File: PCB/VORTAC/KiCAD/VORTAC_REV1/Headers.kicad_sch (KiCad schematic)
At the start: 7 parts, among them J1 DEBUG, J14 918-418K2023S40001, J15 STEPPER, J3 Conn_01x05

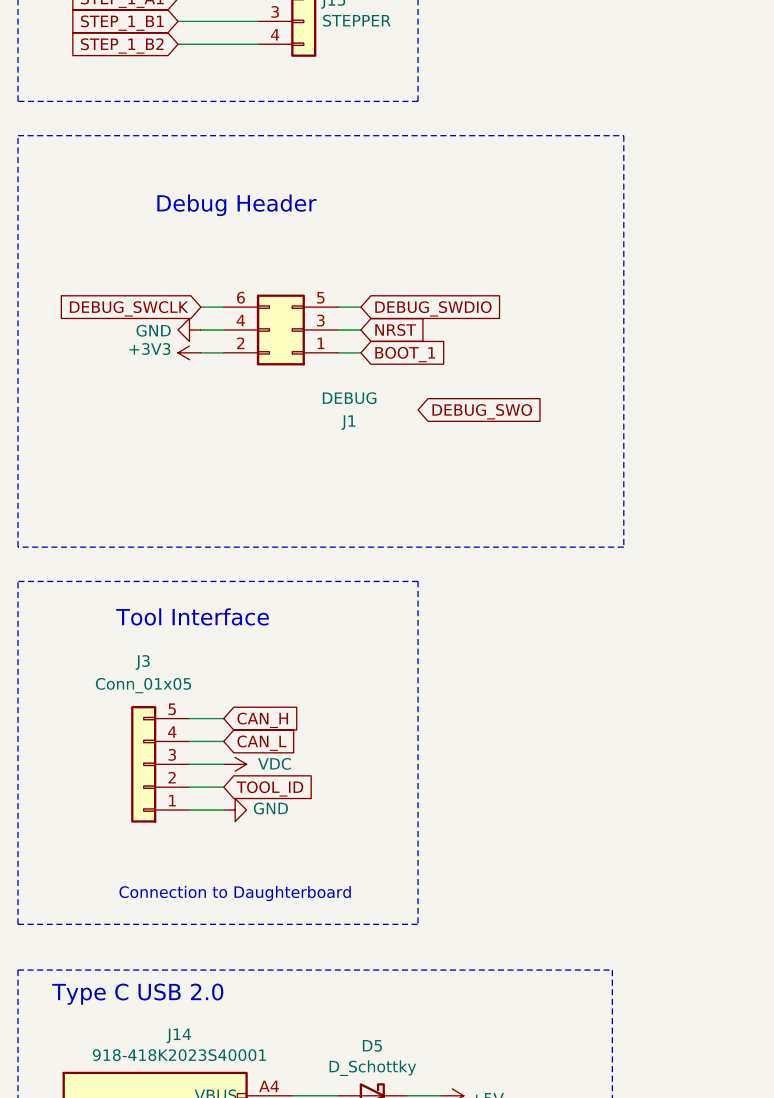
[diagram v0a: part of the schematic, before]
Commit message: Wayollaaaaa
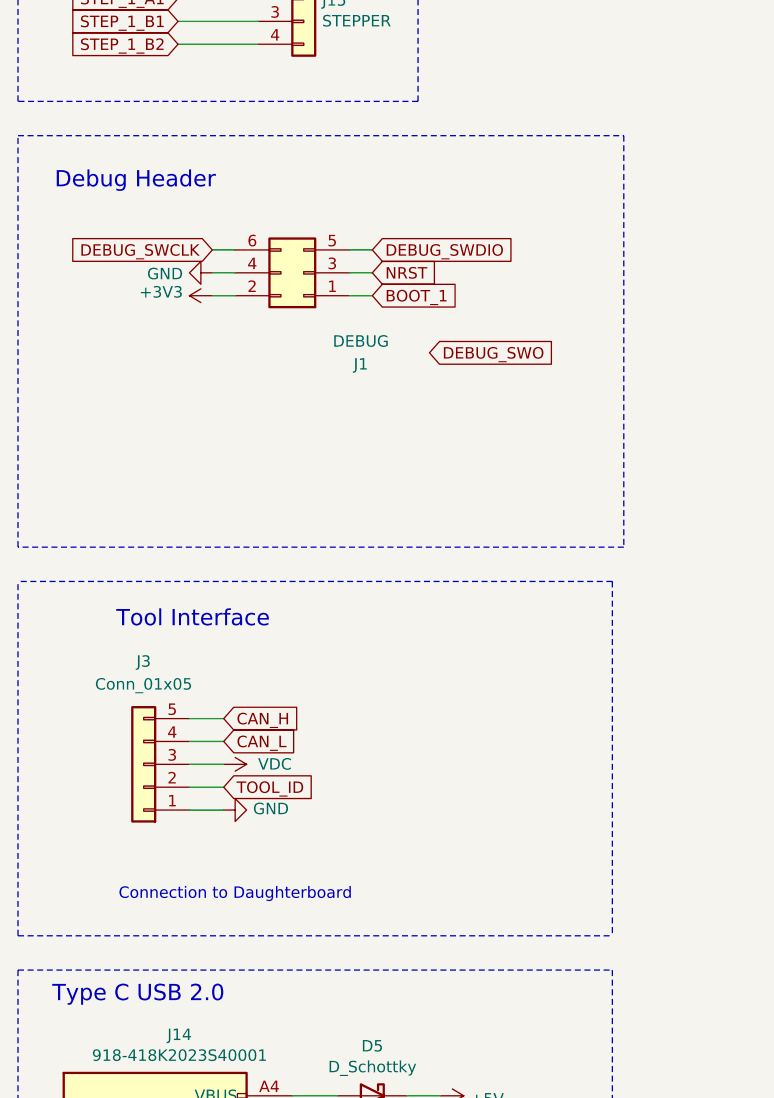
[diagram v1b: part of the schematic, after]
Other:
- moved on the sheet: J1
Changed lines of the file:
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@@
 	(polyline
 		(pts
-			(xy 16.51 132.08) (xy 16.51 93.98)
+			(xy 16.51 133.35) (xy 16.51 93.98)
 		)
 		(stroke
@@
 	(polyline
 		(pts
-			(xy 60.96 93.98) (xy 60.96 132.08)
+			(xy 82.55 93.98) (xy 82.55 133.35)
 		)
 		(stroke
@@
 	(polyline
 		(pts
-			(xy 60.96 93.98) (xy 16.51 93.98)
+			(xy 82.55 93.98) (xy 16.51 93.98)
 		)
 		(stroke
@@
 	(wire
 		(pts
-			(xy 36.83 63.5) (xy 39.37 63.5)
-		)
-		(stroke
-			(width 0)
-			(type default)
-		)
-	)
-	(wire
-		(pts
-			(xy 54.61 68.58) (xy 52.07 68.58)
+			(xy 38.1 57.15) (xy 40.64 57.15)
+		)
+		(stroke
+			(width 0)
+			(type default)
+		)
+	)
+	(wire
+		(pts
+			(xy 55.88 62.23) (xy 53.34 62.23)
 		)
 		(stroke
@@
 	(wire
 		(pts
-			(xy 52.07 63.5) (xy 54.61 63.5)
-		)
-		(stroke
-			(width 0)
-			(type default)
-		)
-	)
-	(wire
-		(pts
-			(xy 39.37 66.04) (xy 36.83 66.04)
+			(xy 53.34 57.15) (xy 55.88 57.15)
+		)
+		(stroke
+			(width 0)
+			(type default)
+		)
+	)
+	(wire
+		(pts
+			(xy 40.64 59.69) (xy 38.1 59.69)
 		)
 		(stroke
@@
 	(wire
 		(pts
-			(xy 52.07 66.04) (xy 54.61 66.04)
+			(xy 53.34 59.69) (xy 55.88 59.69)
 		)
 		(stroke
@@
 	(polyline
 		(pts
-			(xy 16.51 132.08) (xy 60.96 132.08)
+			(xy 16.51 133.35) (xy 82.55 133.35)
 		)
 		(stroke
@@
 	(wire
 		(pts
-			(xy 36.83 68.58) (xy 39.37 68.58)
+			(xy 38.1 62.23) (xy 40.64 62.23)
 		)
 		(stroke
@@
 	(text "Debug Header"
 		(exclude_from_sim no)
-		(at 31.75 53.34 0)
+		(at 20.574 50.546 0)
 		(effects
 			(font
@@
 	(global_label "BOOT_1"
 		(shape input)
-		(at 54.61 68.58 0)
+		(at 55.88 62.23 0)
 		(effects
 			(font
@@
 		)
 		(property "Intersheetrefs" "${INTERSHEET_REFS}"
-			(at 54.61 68.58 0)
+			(at 55.88 62.23 0)
 			(effects
 				(font
@@
 	(global_label "DEBUG_SWDIO"
 		(shape input)
-		(at 54.61 63.5 0)
+		(at 55.88 57.15 0)
 		(effects
 			(font
@@
 		)
 		(property "Intersheetrefs" "${INTERSHEET_REFS}"
-			(at 54.61 63.5 0)
+			(at 55.88 57.15 0)
 			(effects
 				(font
@@
 	(global_label "NRST"
 		(shape input)
-		(at 54.61 66.04 0)
+		(at 55.88 59.69 0)
 		(effects
 			(font
@@
 		)
 		(property "Intersheetrefs" "${INTERSHEET_REFS}"
-			(at 54.61 66.04 0)
+			(at 55.88 59.69 0)
 			(effects
 				(font
@@
 	(global_label "DEBUG_SWO"
 		(shape input)
-		(at 60.96 74.93 0)
+		(at 62.23 68.58 0)
 		(effects
 			(font
@@
 		)
 		(property "Intersheetrefs" "${INTERSHEET_REFS}"
-			(at 60.96 74.93 0)
+			(at 62.23 68.58 0)
 			(effects
 				(font
@@
 	(global_label "DEBUG_SWCLK"
 		(shape input)
-		(at 36.83 63.5 180)
+		(at 38.1 57.15 180)
 		(effects
 			(font
@@
 		)
 		(property "Intersheetrefs" "${INTERSHEET_REFS}"
-			(at 36.83 63.5 0)
+			(at 38.1 57.15 0)
 			(effects
 				(font
@@
 	(symbol
 		(lib_id "Connector_Generic:Conn_02x03_Odd_Even")
-		(at 46.99 66.04 180)
+		(at 48.26 59.69 180)
 		(unit 1)
 		(exclude_from_sim no)
@@
 		(dnp no)
 		(property "Reference" "J1"
-			(at 53.34 76.2 0)
+			(at 54.61 69.85 0)
 			(effects
 				(font
@@
 		)
 		(property "Value" "DEBUG"
-			(at 53.34 73.66 0)
+			(at 54.61 67.31 0)
 			(effects
 				(font
@@
 		)
 		(property "Footprint" "ToolChanger:PinHeader_2x03_P1.27mm_Vertical"
-			(at 46.99 66.04 0)
+			(at 48.26 59.69 0)
 			(effects
 				(font
@@
 		)
 		(property "Datasheet" "~"
-			(at 46.99 66.04 0)
+			(at 48.26 59.69 0)
 			(effects
 				(font
@@
 		)
 		(property "Description" "Generic connector, double row, 02x03, odd/even pin numbering scheme (row 1 odd numbers, row 2 even numbers), script generated (kicad-library-utils/schlib/autogen/connector/)"
-			(at 46.99 66.04 0)
+			(at 48.26 59.69 0)
 			(effects
 				(font
@@
 	(symbol
 		(lib_id "VORTAC-rescue:+3.3V-power")
-		(at 36.83 68.58 90)
+		(at 38.1 62.23 90)
 		(unit 1)
 		(exclude_from_sim no)
@@
 		(dnp no)
 		(property "Reference" "#PWR0160"
-			(at 40.64 68.58 0)
+			(at 41.91 62.23 0)
 			(effects
 				(font
@@
 		)
 		(property "Value" "+3V3"
-			(at 33.5788 68.199 90)
+			(at 34.8488 61.849 90)
 			(effects
 				(font
@@
 		)
 		(property "Footprint" ""
-			(at 36.83 68.58 0)
+			(at 38.1 62.23 0)
 			(effects
 				(font
@@
 		)
 		(property "Datasheet" ""
-			(at 36.83 68.58 0)
+			(at 38.1 62.23 0)
 			(effects
 				(font
@@
 		)
 		(property "Description" ""
-			(at 36.83 68.58 0)
+			(at 38.1 62.23 0)
 			(effects
 				(font
@@
 	(symbol
 		(lib_id "VORTAC-rescue:GND-power")
-		(at 36.83 66.04 270)
+		(at 38.1 59.69 270)
 		(unit 1)
 		(exclude_from_sim no)
@@
 		(dnp no)
 		(property "Reference" "#PWR0161"
-			(at 30.48 66.04 0)
+			(at 31.75 59.69 0)
 			(effects
 				(font
@@
 		)
 		(property "Value" "GND"
-			(at 33.5788 66.167 90)
+			(at 34.8488 59.817 90)
 			(effects
 				(font
@@
 		)
 		(property "Footprint" ""
-			(at 36.83 66.04 0)
+			(at 38.1 59.69 0)
 			(effects
 				(font
@@
 		)
 		(property "Datasheet" ""
-			(at 36.83 66.04 0)
+			(at 38.1 59.69 0)
 			(effects
 				(font
@@
 		)
 		(property "Description" ""
-			(at 36.83 66.04 0)
-			(effects
-				(font
+			(at 38.1 59.69 0)
+			(effects
+				(font

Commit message: Fixed Library stuff
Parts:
- J1: footprint ToolChanger:PinHeader_2x03_P1.27mm_Vertical -> Vortac:PinHeader_2x03_P1.27mm_Vertical
- J14: footprint ToolChanger:USB-C-TH_HANBO_MC-118LD-H65 -> Vortac:USB-C-TH_HANBO_MC-118LD-H65
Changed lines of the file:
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@@
 			)
 		)
-		(property "Footprint" "ToolChanger:USB-C-TH_HANBO_MC-118LD-H65"
+		(property "Footprint" "Vortac:USB-C-TH_HANBO_MC-118LD-H65"
 			(at 35.56 166.37 0)
 			(effects
@@
 			)
 		)
-		(property "Footprint" "ToolChanger:PinHeader_2x03_P1.27mm_Vertical"
+		(property "Footprint" "Vortac:PinHeader_2x03_P1.27mm_Vertical"
 			(at 48.26 59.69 0)
 			(effects
